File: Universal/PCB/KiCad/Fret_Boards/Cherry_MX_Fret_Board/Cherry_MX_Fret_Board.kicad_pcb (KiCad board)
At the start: 2 copper layers, 121 x 24 mm, 24 parts, among them SW1 MX_SW_HS, SW2 MX_SW_HS, SW3 MX_SW_HS, SW4 MX_SW_HS, SW5 MX_SW_HS

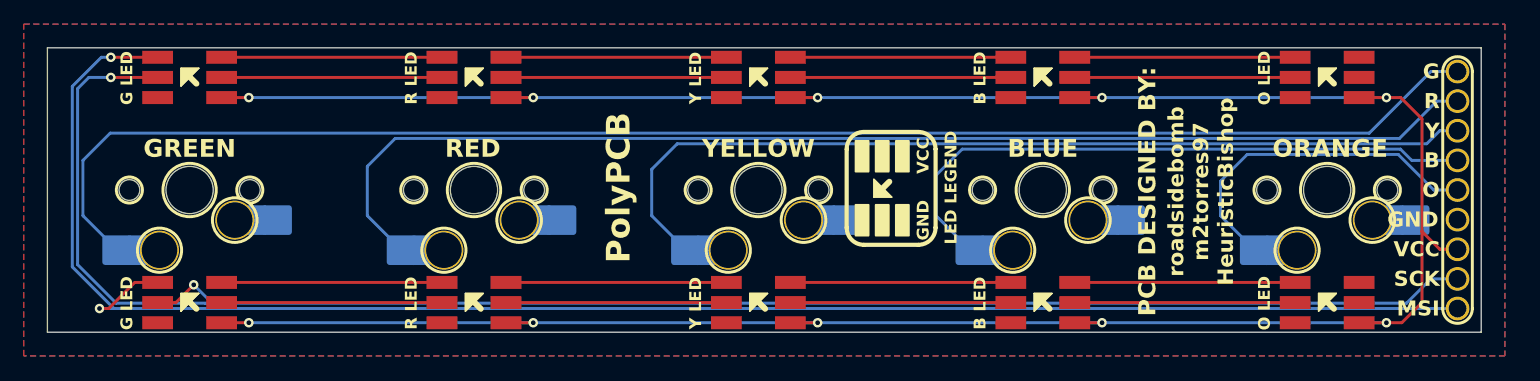
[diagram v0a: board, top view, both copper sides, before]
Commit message: updated the MX fret board
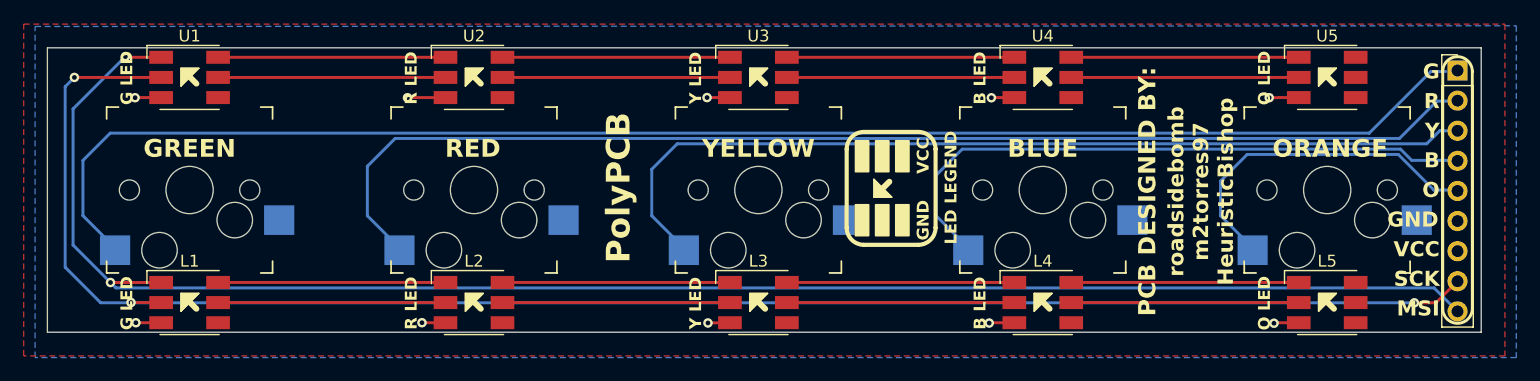
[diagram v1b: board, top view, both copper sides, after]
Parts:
- removed ?: R, 
- removed ? (x4): , 
- removed ?: G, 
- removed ?: B, 
- removed ?: O, 
- removed ?: GND, 
- added J1: Conn_01x09_Pin, Connector_PinHeader_2.54mm:PinHeader_1x09_P2.54mm_Vertical, F.Cu at (181.0, 79.9)
- L1, U1: renamed from D1; footprint Controller_Inputs:LED_RGB_5050_DOTSTAR -> LED_SMD:LED_RGB_5050-6
- L2, U2: renamed from D2; footprint Controller_Inputs:LED_RGB_5050_DOTSTAR -> LED_SMD:LED_RGB_5050-6
- L3, U3: renamed from D3; footprint Controller_Inputs:LED_RGB_5050_DOTSTAR -> LED_SMD:LED_RGB_5050-6
- L4, U4: renamed from D4; footprint Controller_Inputs:LED_RGB_5050_DOTSTAR -> LED_SMD:LED_RGB_5050-6
- L5, U5: renamed from D5; footprint Controller_Inputs:LED_RGB_5050_DOTSTAR -> LED_SMD:LED_RGB_5050-6
- SW1, SW2, SW3, SW4, SW5: value MX_SW_HS -> SW_HS; footprint marbastlib-mx:SW_MX_HS_1u -> Minibar:Kailh_Hotswap_MX; moved to F.Cu
- turned SW1 to 180 degrees
- turned SW2 to 180 degrees
- turned SW3 to 180 degrees
- turned SW4 to 180 degrees
- turned SW5 to 180 degrees
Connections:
- net led_mosi renamed fret_mosi
- net led_sck renamed fret_sck
- L1 pad 5: Net-(D1-CO) -> Net-(L1-CO)
- L1 pad 6: Net-(D1-DO) -> Net-(L1-DO)
- L2 pad 1: Net-(D1-DO) -> Net-(L1-DO)
- L2 pad 2: Net-(D1-CO) -> Net-(L1-CO)
- L2 pad 5: Net-(D2-CO) -> Net-(L2-CO)
- L2 pad 6: Net-(D2-DO) -> Net-(L2-DO)
- L3 pad 1: Net-(D2-DO) -> Net-(L2-DO)
- L3 pad 2: Net-(D2-CO) -> Net-(L2-CO)
- L3 pad 5: Net-(D3-CO) -> Net-(L3-CO)
- L3 pad 6: Net-(D3-DO) -> Net-(L3-DO)
- L4 pad 1: Net-(D3-DO) -> Net-(L3-DO)
- L4 pad 2: Net-(D3-CO) -> Net-(L3-CO)
- L4 pad 5: Net-(D4-CO) -> Net-(L4-CO)
- L4 pad 6: Net-(D4-DO) -> Net-(L4-DO)
- L5 pad 1: Net-(D4-DO) -> Net-(L4-DO)
- L5 pad 2: Net-(D4-CO) -> Net-(L4-CO)
- L5 pad 5: unconnected-(D5-CO-Pad5) -> unconnected-(L5-CO-Pad5)
- L5 pad 6: unconnected-(D5-DO-Pad6) -> unconnected-(L5-DO-Pad6)
- SW1 pad 1: GND -> Green
- SW1 pad 2: Green -> GND
- SW2 pad 1: GND -> Red
- SW2 pad 2: Red -> GND
- SW3 pad 1: GND -> Yellow
- SW3 pad 2: Yellow -> GND
- SW4 pad 1: GND -> Blue
- SW4 pad 2: Blue -> GND
- SW5 pad 1: GND -> Orange
- SW5 pad 2: Orange -> GND
- U1 pad 5: Net-(D1-CO) -> Net-(U1-CO)
- U1 pad 6: Net-(D1-DO) -> Net-(U1-DO)
- U2 pad 1: Net-(D1-DO) -> Net-(U1-DO)
- U2 pad 2: Net-(D1-CO) -> Net-(U1-CO)
- U2 pad 5: Net-(D2-CO) -> Net-(U2-CO)
- U2 pad 6: Net-(D2-DO) -> Net-(U2-DO)
- U3 pad 1: Net-(D2-DO) -> Net-(U2-DO)
- U3 pad 2: Net-(D2-CO) -> Net-(U2-CO)
- U3 pad 5: Net-(D3-CO) -> Net-(U3-CO)
- U3 pad 6: Net-(D3-DO) -> Net-(U3-DO)
- U4 pad 1: Net-(D3-DO) -> Net-(U3-DO)
- U4 pad 2: Net-(D3-CO) -> Net-(U3-CO)
- U4 pad 5: Net-(D4-CO) -> Net-(U4-CO)
- U4 pad 6: Net-(D4-DO) -> Net-(U4-DO)
- U5 pad 1: Net-(D4-DO) -> Net-(U4-DO)
- U5 pad 2: Net-(D4-CO) -> Net-(U4-CO)
- U5 pad 5: unconnected-(D5-CO-Pad5) -> unconnected-(U5-CO-Pad5)
- U5 pad 6: unconnected-(D5-DO-Pad6) -> unconnected-(U5-DO-Pad6)
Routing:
- net VCC: track 241.9 -> 0.00 mm, vias 10 -> 0
- net Net-(D4-DO): track 37.2 -> 0.00 mm
- net Net-(D4-CO): track 37.2 -> 0.00 mm
- net Net-(D3-DO): track 37.2 -> 0.00 mm
- net Net-(D3-CO): track 37.2 -> 0.00 mm
- net Net-(D2-DO): track 37.2 -> 0.00 mm
- net Net-(D2-CO): track 37.2 -> 0.00 mm
- net Net-(D1-DO): track 37.2 -> 0.00 mm
- net Net-(D1-CO): track 37.2 -> 0.00 mm
- net GND: track 0.00 -> 22.3 mm, vias 0 -> 10
- net Net-(U4-DO): track 0.00 -> 18.6 mm
- net Net-(U4-CO): track 0.00 -> 18.6 mm
- net Net-(L4-DO): track 0.00 -> 18.6 mm
- net Net-(L4-CO): track 0.00 -> 18.6 mm
- net Net-(U3-DO): track 0.00 -> 18.6 mm
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- added copper zone on F.Cu, net VCC
- removed copper zone on F.Cu, net GND
